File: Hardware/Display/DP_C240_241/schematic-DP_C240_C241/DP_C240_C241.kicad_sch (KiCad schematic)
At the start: 16 parts

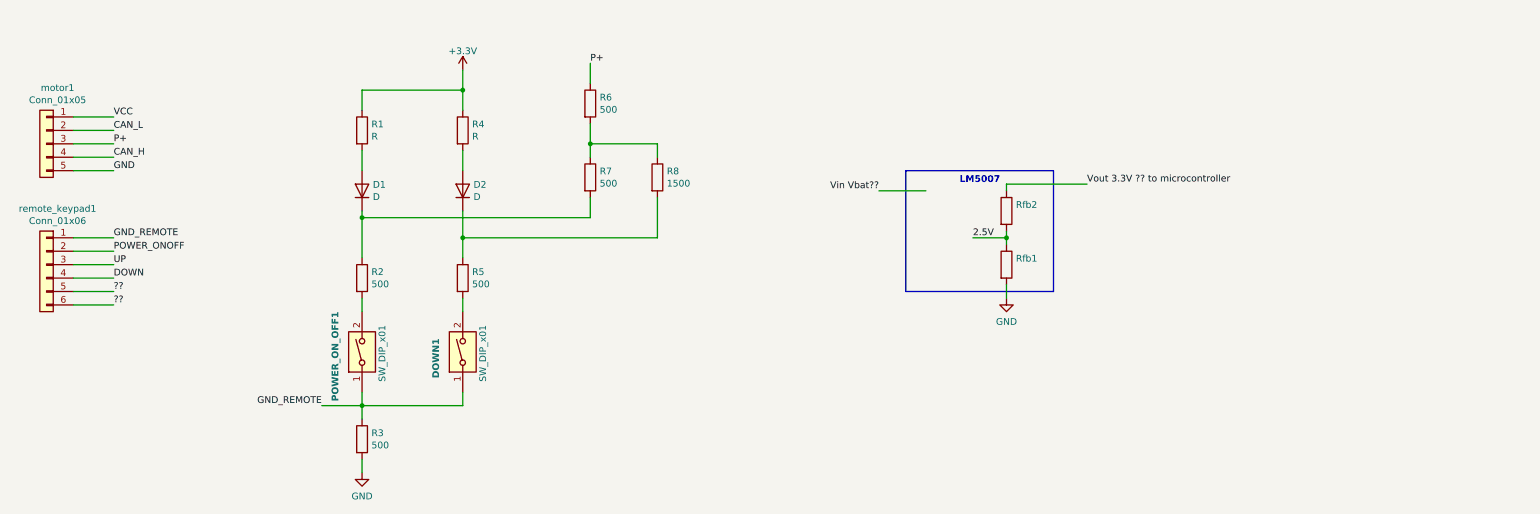
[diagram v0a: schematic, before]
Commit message: WIP schematic
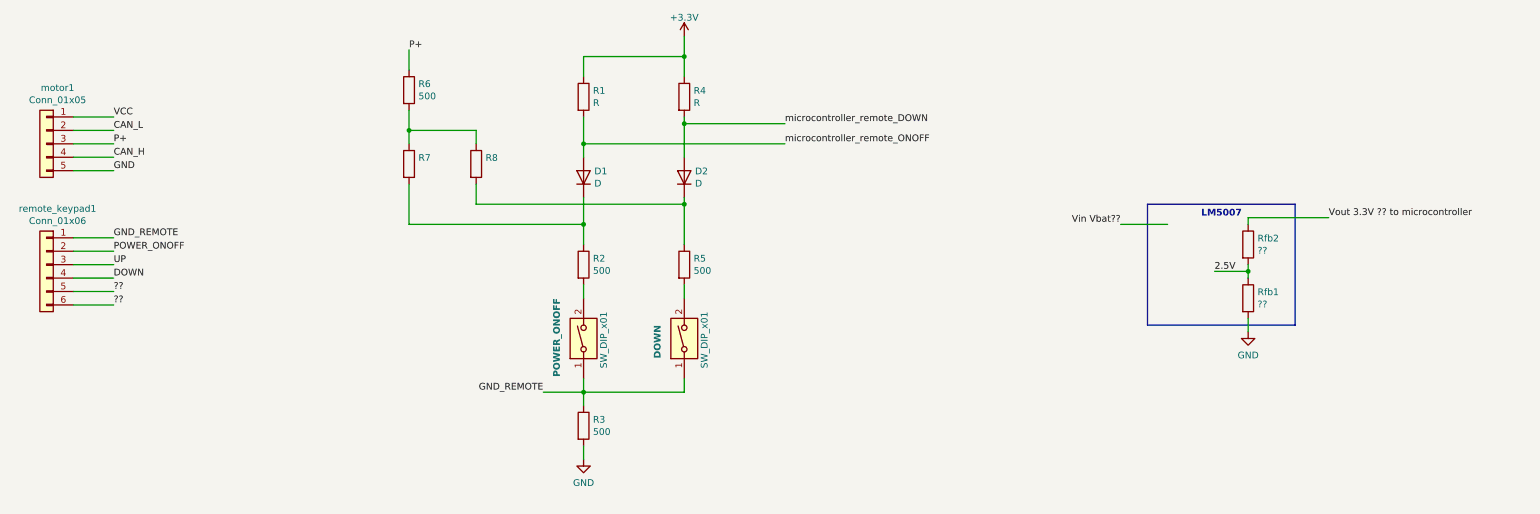
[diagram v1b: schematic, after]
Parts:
- R7: value 500 -> (none)
- R8: value 1500 -> (none)
- Rfb1, Rfb2: value (none) -> ??
- renumbered DOWN1 to DOWN, POWER_ON_OFF1 to POWER_ONOFF
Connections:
- net microcontroller_remote_ONOFF: now reaches D1.2 (A), R1.2
- net microcontroller_remote_DOWN: now reaches D2.2 (A), R4.2
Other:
- moved on the sheet: D1, D2, DOWN, POWER_ONOFF, R1, R2, R3, R4, R5, R6, R7, R8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
